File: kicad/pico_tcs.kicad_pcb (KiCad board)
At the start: 2 copper layers, 101.3 x 66.5 mm, 14 parts, among them J1 TCS In, J2 Conn_01x20_Male, J3 Conn_01x20_Male, J4 Keypad, J5 Display, U1 L7805, U2 ULN2003

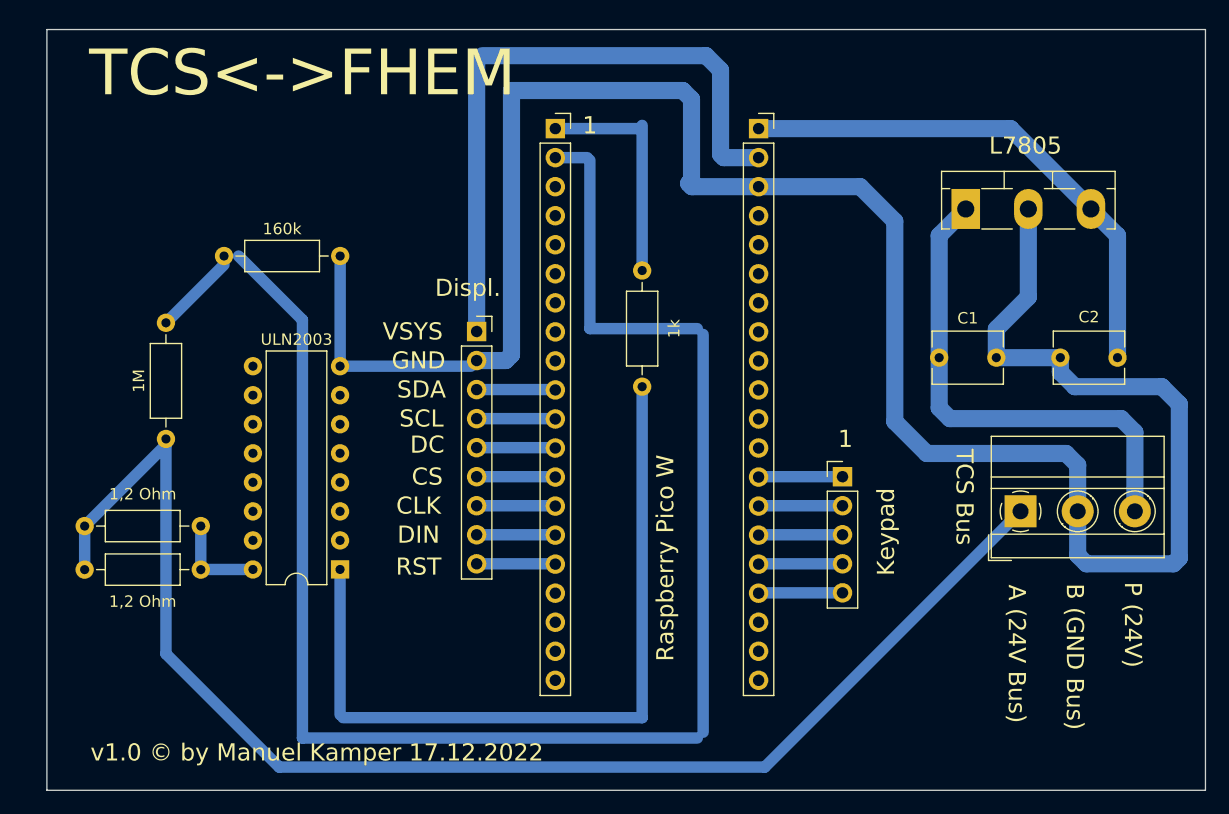
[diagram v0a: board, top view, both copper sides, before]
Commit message: Dateien hochladen nach „kicad“
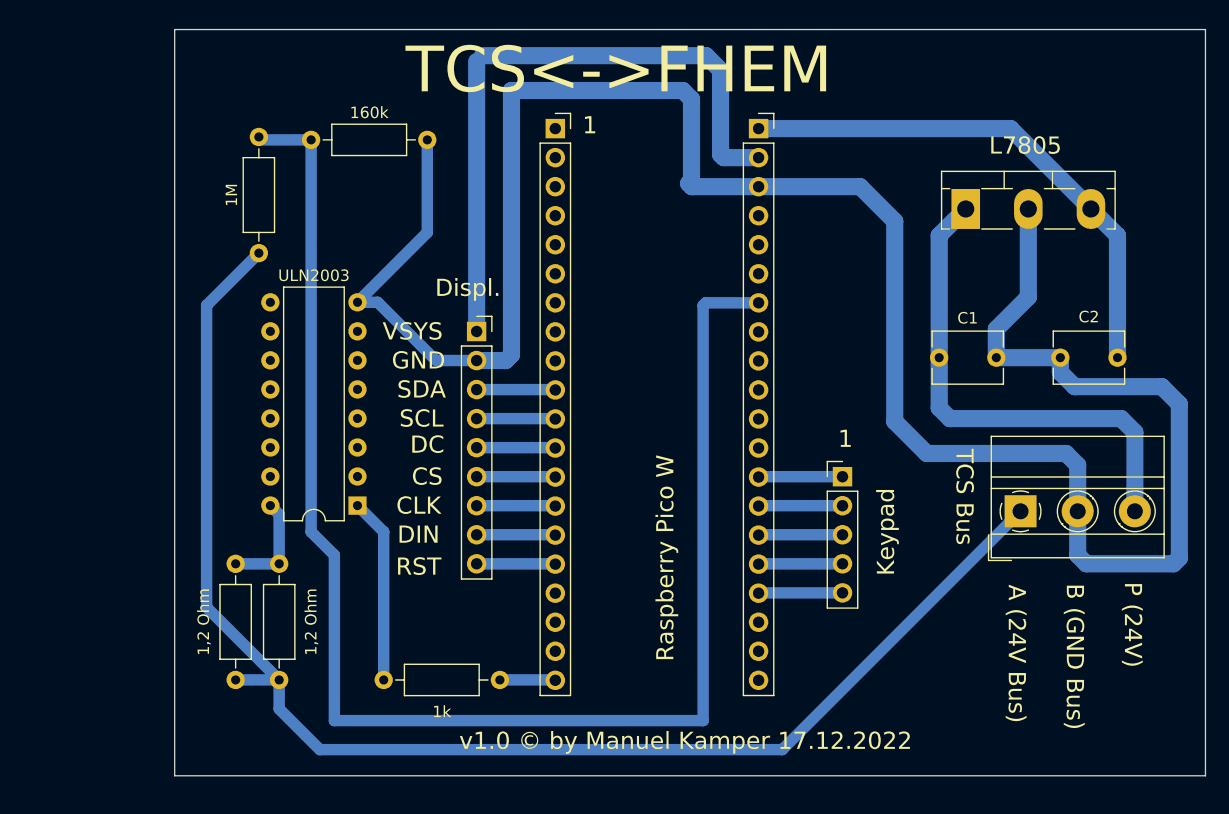
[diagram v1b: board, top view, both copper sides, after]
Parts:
- moved R5 37.9 mm to (140.0, 115.6), turned to 180 degrees
- moved R3 18.2 mm to (118.9, 68.1)
- moved R4 12.7 mm to (133.6, 68.3)
- moved R1 6.88 mm to (120.7, 105.4), turned to -90 degrees
- moved U2 5.79 mm to (127.5, 100.3)
- moved R2 4.49 mm to (116.8, 105.4), turned to -90 degrees
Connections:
- J2 pad 1: Net-(J2-Pad1) -> unconnected-(J2-Pad1)
- J2 pad 2: Net-(J2-Pad2) -> unconnected-(J2-Pad2)
- J2 pad 20: unconnected-(J2-Pad20) -> Net-(J2-Pad20)
- J3 pad 7: unconnected-(J3-Pad7) -> Net-(R3-Pad1)
- R3 pad 1: Net-(J2-Pad2) -> Net-(R3-Pad1)
- R4 pad 2: Net-(J2-Pad2) -> Net-(R3-Pad1)
- R5 pad 1: Net-(J2-Pad1) -> Net-(J2-Pad20)
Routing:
- net Net-(J2-Pad2): track 151.7 -> 0.00 mm
- net Net-(R3-Pad1): track 0.00 -> 129.8 mm
- net Net-(R5-Pad2): track 68.2 -> 16.2 mm
- net Net-(J2-Pad1): track 20.4 -> 0.00 mm
- net GND: track 189.6 -> 198.5 mm
- net Net-(J2-Pad20): track 0.00 -> 4.86 mm
- net Net-(J1-Pad1): track 121.3 -> 123.2 mm
- net Net-(R1-Pad1): track 8.37 -> 9.22 mm
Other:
- board size 101.3 x 66.5 mm -> 90.2 x 65.3 mm
